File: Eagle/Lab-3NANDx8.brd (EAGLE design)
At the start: 160 x 20 mm, 100 parts, among them CN0 HD4, CN1 HD4, CN2 HD4, CN3 HD4, CN4 HD4, CN5 HD4, CN6 HD4, CN7 HD4, CN8 HD4, CN9 HD4, Q1 2N3904-1, Q2 2N3904-1, Q3 2N3904-1, Q4 2N3904-1, Q5 2N3904-1, Q6 2N3904-1, Q7 2N3904-1, Q8 2N3904-1

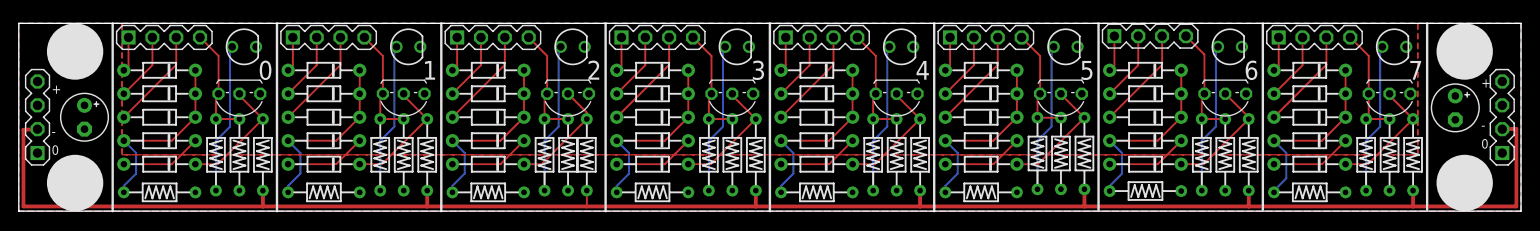
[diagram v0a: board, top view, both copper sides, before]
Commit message: General flush of files
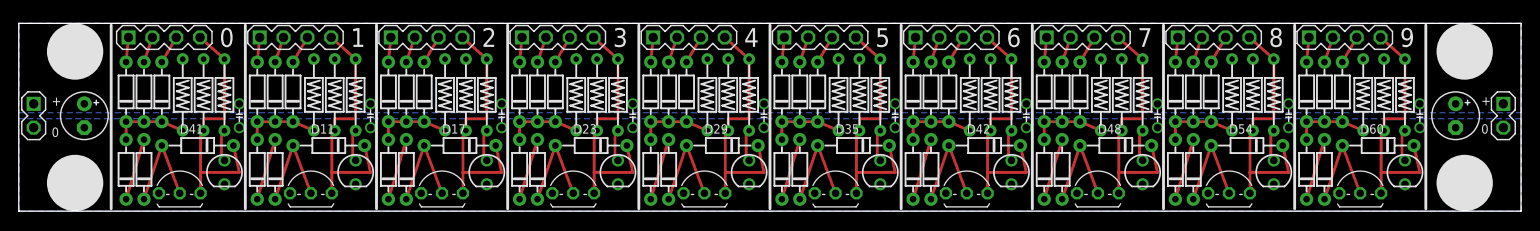
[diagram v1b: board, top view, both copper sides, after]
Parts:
- removed CN0, CN8: HD4, SmallRoomLabs_ConSwitch:HD4
- removed R31, R32: R1/8-7.6MM, SmallRoomLabs_Discrete:R0125-7.6
- added CN10: HD2, SmallRoomLabs_ConSwitch:HD2
- added CN11, CN12, CN14: HD4, SmallRoomLabs_ConSwitch:HD4
- added D41, D42, D48, D54, D60: DIODE-7.6, SmallRoomLabs_Semiconductor:DO35-7.6
- added D43, D44, D45, D46, D47, D49, D50, D51, D52, D53, D55, D56, D57, D58, D59: DIODE-6.3, SmallRoomLabs_Semiconductor:DO35-6.3
- added LD10, LD9: LED3MM, SmallRoomLabs_Led:3MM
- added Q10, Q9: 2N3904-1, SmallRoomLabs_Semiconductor:TO92BH
- CN6: value HD4 -> HD2; device SmallRoomLabs_ConSwitch:HD4 -> SmallRoomLabs_ConSwitch:HD2
- D1, D10, D12, D13, D14, D15, D16, D18, D19, D2, D20, D21, D22, D24, D25, D26, D27, D28, D3, D30, D31, D32, D33, D34, D36, D37, D38, D39, D4, D40, D5, D6, D7, D8, D9: value DIODE-7.6 -> DIODE-6.3; device SmallRoomLabs_Semiconductor:DO35-7.6 -> SmallRoomLabs_Semiconductor:DO35-6.3
- moved CN6 156.4 mm to (1.59, 10.2), turned to 270 degrees
- moved CN5 59.3 mm to (127.3, 18.5)
- moved CN9 52.7 mm to (85.3, 18.5)
- moved CN7 45.6 mm to (57.4, 18.5)
- moved D39 42.4 mm to (95.2, 4.45), turned to 270 degrees
- moved D36 42.3 mm to (95.2, 12.7), turned to 270 degrees
- moved D40 40.3 mm to (97.2, 4.45), turned to 270 degrees
- moved D37 40.3 mm to (97.2, 12.7), turned to 270 degrees
- moved D33 39.1 mm to (81.3, 4.45), turned to 270 degrees
- moved D38 38.5 mm to (99.1, 12.7), turned to 270 degrees
- moved D34 36.9 mm to (83.2, 4.45), turned to 270 degrees
- moved D31 36.9 mm to (83.2, 12.7), turned to 270 degrees
- moved D27 36.1 mm to (67.3, 4.45), turned to 270 degrees
- moved D32 34.9 mm to (85.1, 12.7), turned to 270 degrees
- moved D28 33.7 mm to (69.2, 4.45), turned to 270 degrees
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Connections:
- removed net N$53 (its old number): D34.C, D35.A
- removed net V-: CN0.P$2, CN6.P$2, R10.1, R14.1, R18.1, R2.1, R22.1, R26.1, R30.1, R6.1
- new net N$61: D46.C, D47.A
- new net N$65: CN5.P$1, D49.A
- new net N$66: CN5.P$2, D50.A
- new net N$67: CN5.P$3, D51.A
- new net N$68: D49.C, D50.C, D51.C, D52.A, R25.1
- new net N$69: D52.C, D53.A
- new net N$70: D53.C, D54.A, Q9.2
- new net N$71: CN5.P$4, D54.C, Q9.3, R26.1, R27.2
- new net N$72: LD9.A, R27.1
- new net N$73: CN14.P$1, D55.A
- new net N$74: CN14.P$2, D56.A
- new net N$75: CN14.P$3, D57.A
- new net N$76: D55.C, D56.C, D57.C, D58.A, R28.1
- new net N$77: D58.C, D59.A
- new net N$78: D59.C, D60.A, Q10.2
- new net N$79: CN14.P$4, D60.C, Q10.3, R29.1, R30.2
- new net N$80: LD10.A, R30.1
- net GND: now also CN10.P$2, CN6.P$2, LD10.C, LD9.C, Q10.1, Q9.1; no longer CN0.P$1, CN6.P$1
- net N$12: now also R2.1; no longer R5.1
- net N$14: now also D11.A; no longer R6.2
- net N$15: now also D11.C, R5.1, R6.2; no longer R7.1, R8.2
- net N$16: now also R6.1; no longer R8.1
- net N$17: now also D12.A; no longer D11.A
- net N$18: now also D13.A; no longer D12.A
- net N$19: now also D14.A; no longer D13.A
- net N$20: now also D14.C, D15.A, R7.1; no longer D11.C, D14.A, R9.1
- net N$21: now also D15.C, D16.A; no longer D14.C, D15.A
- net N$22: now also D16.C, D17.A; no longer D15.C, R10.2
- net N$23: now also D17.C, R8.1, R9.2; no longer R11.1, R12.2
- net N$24: now also R9.1; no longer R12.1
- net N$25: now also CN7.P$1, D18.A; no longer CN5.P$1, D16.A
- net N$26: now also CN7.P$2, D19.A; no longer CN5.P$2, D17.A
- net N$27: now also CN7.P$3, D20.A; no longer CN5.P$3, D18.A
- net N$28: now also D19.C, D20.C, D21.A, R10.1; no longer D16.C, D17.C, D19.A, R13.1
- net N$29: now also D21.C, D22.A; no longer D19.C, D20.A
- net N$30: now also D22.C, D23.A; no longer D20.C, R14.2
- net N$31: now also CN7.P$4, D23.C, R11.1, R12.2; no longer CN5.P$4, R15.1, R16.2
- net N$32: now also R12.1; no longer R16.1
- net N$33: now also D24.A; no longer D21.A
- net N$34: now also D25.A; no longer D22.A
- net N$35: now also D26.A; no longer D23.A
- net N$36: now also D24.C, D25.C, D26.C, D27.A, R13.1; no longer D21.C, D22.C, D23.C, D24.A, R17.1
- net N$37: now also D27.C, D28.A; no longer D24.C, D25.A
- net N$38: now also D28.C, D29.A; no longer D25.C, R18.2
- net N$39: now also D29.C, R14.1, R15.2; no longer R19.1, R20.2
- net N$40: now also R15.1; no longer R20.1
- net N$41: now also CN9.P$1, D30.A; no longer CN7.P$1, D26.A
- net N$42: now also CN9.P$2, D31.A; no longer CN7.P$2, D27.A
- net N$43: now also CN9.P$3, D32.A; no longer CN7.P$3, D28.A
- net N$44: now also D30.C, D31.C, D32.C, D33.A, R16.1; no longer D26.C, D27.C, D28.C, D29.A, R21.1
- net N$45: now also D33.C, D34.A; no longer D29.C, D30.A
- net N$46: now also D34.C, D35.A; no longer D30.C, R22.2
- net N$47: now also CN9.P$4, D35.C, R17.1, R18.2; no longer CN7.P$4, R23.1, R24.2
- net N$48: now also R18.1; no longer R24.1
- net N$49: now also CN11.P$1, D36.A; no longer CN8.P$1, D31.A
- net N$50: now also CN11.P$2, D37.A; no longer CN8.P$2, D32.A
- net N$51: now also CN11.P$3, D38.A; no longer CN8.P$3, D33.A
- net N$52: now also D36.C, D37.C, D38.C, D39.A, R19.1; no longer D31.C, D32.C, D33.C, D34.A, R25.1
- net N$54: now also D40.C, D42.A; no longer D35.C, R26.2
- net N$55: now also CN11.P$4, D42.C, R20.1, R21.2; no longer CN8.P$4, R27.1, R28.2
- net N$56: now also R21.1; no longer R28.1
- net N$57: now also CN12.P$1, D43.A; no longer CN9.P$1, D36.A
- net N$58: now also CN12.P$2, D44.A; no longer CN9.P$2, D37.A
- net N$59: now also CN12.P$3, D45.A; no longer CN9.P$3, D38.A
- net N$6: now also D41.A; no longer R2.2
- net N$60: now also D43.C, D44.C, D45.C, D46.A, R22.1; no longer D36.C, D37.C, D38.C, D39.A, R29.1
- net N$62: now also D47.C, D48.A; no longer D40.C, R30.2
- net N$63: now also CN12.P$4, D48.C, R23.1, R24.2; no longer CN9.P$4, R31.1, R32.2
- net N$64: now also R24.1; no longer R32.1
- net N$8: now also D41.C
- net V+: now also CN10.P$1, CN6.P$1, R10.2, R14.2, R16.2, R2.2, R20.2, R22.2, R26.2, R28.2, R8.2; no longer CN0.P$4, CN6.P$4, R15.2, R21.2, R27.2, R31.2, R9.2
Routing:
- net V-: track 192.1 -> 0.00 mm
- net N$79: track 0.00 -> 27.1 mm
- net N$71: track 0.00 -> 27.1 mm
- net N$47: track 12.0 -> 27.1 mm
- net N$63: track 12.1 -> 27.1 mm
- net N$31: track 12.1 -> 27.1 mm
- net N$8: track 12.1 -> 27.1 mm
- net N$23: track 12.1 -> 27.1 mm
- net N$15: track 12.1 -> 27.1 mm
- net N$39: track 12.1 -> 27.1 mm
- net N$55: track 12.3 -> 27.1 mm
- net N$40: track 16.0 -> 3.44 mm
- net N$24: track 16.0 -> 3.44 mm
- net N$16: track 16.0 -> 3.44 mm
- net N$7: track 16.0 -> 3.44 mm
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- added copper zone on layer 16, net V+
- removed copper zone on layer 1, net GND
- removed copper zone on layer 1, net V+
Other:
- board text added: "3NAND*10"
- board text added: "8"
- board text added: "9"
- board text removed: "3NAND*8"
